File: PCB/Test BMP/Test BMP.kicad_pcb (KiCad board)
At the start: 2 copper layers, 14 x 8 mm, 5 parts, among them J1 4 pins socket, J2 4 pins socket, U1 BMP581

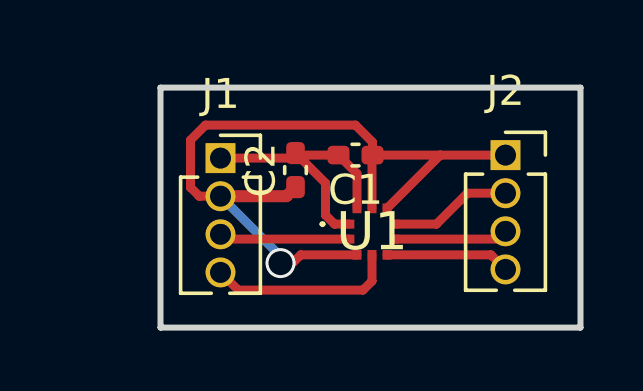
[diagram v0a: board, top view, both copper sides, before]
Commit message: gbr
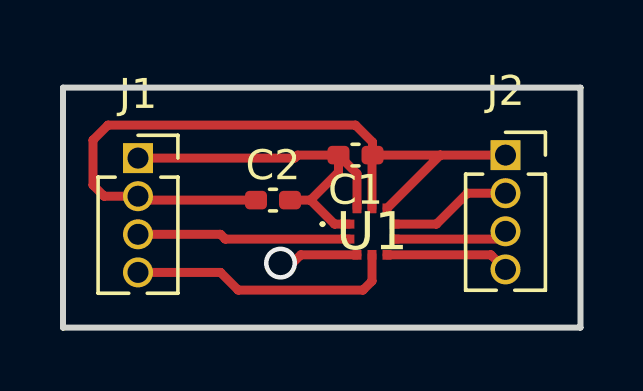
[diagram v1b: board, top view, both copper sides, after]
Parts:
- moved J1 2.75 mm to (135.2, 87.6)
- moved C2 1.25 mm to (139.8, 89.0), turned to 0 degrees
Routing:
- net Net-(J1-Pin_1): track 9.47 -> 13.0 mm
- net Net-(J1-Pin_3): track 4.37 -> 7.12 mm
- net Net-(J1-Pin_4): track 6.29 -> 9.04 mm
- net Net-(J1-Pin_2): track 26.7 -> 29.0 mm
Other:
- board size 14 x 8 mm -> 17.2 x 8 mm
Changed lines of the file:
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@@
 		(filling no)
 		(pcbplotparams
-			(layerselection 0x00000000_00000000_55555555_5755f5ff)
-			(plot_on_all_layers_selection 0x00000000_00000000_00000000_00000000)
+			(layerselection 0x00000000_00000000_55555555_57555555)
+			(plot_on_all_layers_selection 0x00000000_00000000_00000000_02000000)
 			(disableapertmacros no)
 			(usegerberextensions no)
@@
 			(outputformat 1)
 			(mirror no)
-			(drillshape 1)
+			(drillshape 0)
 			(scaleselection 1)
 			(outputdirectory "")
@@
 	(footprint "Capacitor_SMD:C_0402_1005Metric_Pad0.74x0.62mm_HandSolder"
 		(layer "F.Cu")
-		(at 140.5 88 90)
+		(at 139.75 89)
 		(descr "Capacitor SMD 0402 (1005 Metric), square (rectangular) end terminal, IPC-7351 nominal with elongated pad for handsoldering. (Body size source: IPC-SM-782 page 76, https://www.pcb-3d.com/wordpress/wp-content/uploads/ipc-sm-782a_amendment_1_and_2.pdf)")
 		(tags "capacitor handsolder")
 		(property "Reference" "C2"
-			(at 0 -1.16 90)
+			(at 0 -1.16 0)
 			(layer "F.SilkS")
 			(effects
@@
 		)
 		(property "Value" "C"
-			(at 0 1.16 90)
+			(at 0 1.16 0)
 			(layer "F.Fab")
 			(effects
@@
 		)
 		(property "Datasheet" ""
-			(at 0 0 90)
+			(at 0 0 0)
 			(layer "F.Fab")
 			(hide yes)
@@
 		)
 		(property "Description" "Unpolarized capacitor"
-			(at 0 0 90)
+			(at 0 0 0)
 			(layer "F.Fab")
 			(hide yes)
@@
 		)
 		(property "KiLib_Generator" "SMD_2terminal_chip_molded"
-			(at 0 0 90)
+			(at 0 0 0)
 			(layer "F.SilkS")
 			(hide yes)
@@
 		)
 		(fp_text user "${REFERENCE}"
-			(at 0 0 90)
+			(at 0 0 0)
 			(layer "F.Fab")
 			(effects
@@
 		)
 		(pad "1" smd roundrect
-			(at -0.5675 0 90)
+			(at -0.5675 0)
 			(size 0.735 0.62)
 			(layers "F.Cu" "F.Mask" "F.Paste")
@@
 		)
 		(pad "2" smd roundrect
-			(at 0.5675 0 90)
+			(at 0.5675 0)
 			(size 0.735 0.62)
 			(layers "F.Cu" "F.Mask" "F.Paste")
@@
 	(footprint "Bibliotheque_Projet:4 pins socket"
 		(layer "F.Cu")
-		(at 138 87.6)
+		(at 135.25 87.6)
 		(descr "Through hole straight socket strip, 1x04, 1.27mm pitch, single row (from Kicad 4.0.7), script generated")
 		(tags "Through hole socket strip THT 1x04 1.27mm single row")
@@
 	)
 	(gr_rect
-		(start 136 85.25)
+		(start 132.75 85.25)
 		(end 150 93.25)
 		(stroke
@@
 	)
 	(segment
-		(start 140.5675 87.5)
-		(end 140.5 87.4325)
-		(width 0.2)
-		(layer "F.Cu")
-		(net "Net-(J1-Pin_1)")
-	)
-	(segment
-		(start 140.3325 87.6)
-		(end 140.5 87.4325)
-		(width 0.2)
+		(start 141 89)
+		(end 141.9325 88.0675)
+		(width 0.3)
 		(layer "F.Cu")
 		(net "Net-(J1-Pin_1)")
@@
 	)
 	(segment
-		(start 141.5 88.4325)
-		(end 140.5 87.4325)
+		(start 141 89)
+		(end 140.3175 89)
 		(width 0.3)
 		(layer "F.Cu")
@@
 	)
 	(segment
-		(start 138 87.6)
-		(end 140.3325 87.6)
+		(start 140.4675 87.6)
+		(end 135.25 87.6)
 		(width 0.3)
 		(layer "F.Cu")
@@
 	(segment
 		(start 141.8 89.8)
-		(end 141.5 89.5)
+		(end 141 89)
 		(width 0.3)
 		(layer "F.Cu")
@@
 	)
 	(segment
-		(start 141.5 89.5)
-		(end 141.5 88.4325)
+		(start 140.5675 87.5)
+		(end 140.4675 87.6)
+		(width 0.3)
+		(layer "F.Cu")
+		(net "Net-(J1-Pin_1)")
+	)
+	(segment
+		(start 141.9325 88.0675)
+		(end 141.9325 87.5)
 		(width 0.3)
 		(layer "F.Cu")
@@
 	)
 	(segment
+		(start 138 90.14)
+		(end 135.25 90.14)
+		(width 0.3)
+		(layer "F.Cu")
+		(net "Net-(J1-Pin_3)")
+	)
+	(segment
+		(start 142.3 90.3)
+		(end 138.16 90.3)
+		(width 0.3)
+		(layer "F.Cu")
+		(net "Net-(J1-Pin_3)")
+	)
+	(segment
 		(start 138.16 90.3)
 		(end 138 90.14)
-		(width 0.2)
+		(width 0.3)
 		(layer "F.Cu")
 		(net "Net-(J1-Pin_3)")
 	)
 	(segment
-		(start 142.3 90.3)
-		(end 138.16 90.3)
-		(width 0.3)
-		(layer "F.Cu")
-		(net "Net-(J1-Pin_3)")
-	)
-	(segment
-		(start 140.1975 88.87)
-		(end 140.5 88.5675)
-		(width 0.4)
+		(start 133.75 88.5)
+		(end 134.12 88.87)
+		(width 0.3)
 		(layer "F.Cu")
 		(net "Net-(J1-Pin_2)")
@@
 	)
 	(segment
-		(start 143.0675 87.5)
-		(end 143.0675 87.0675)
-		(width 0.3)
-		(layer "F.Cu")
-		(net "Net-(J1-Pin_2)")
-	)
-	(segment
-		(start 137 87)
-		(end 137 88.577106)
-		(width 0.3)
-		(layer "F.Cu")
-		(net "Net-(J1-Pin_2)")
-	)
-	(segment
-		(start 137.5 86.5)
-		(end 137 87)
+		(start 143.0675 87.0675)
+		(end 142.5 86.5)
+		(width 0.3)
+		(layer "F.Cu")
+		(net "Net-(J1-Pin_2)")
+	)
+	(segment
+		(start 134.25 86.5)
+		(end 133.75 87)
+		(width 0.3)
+		(layer "F.Cu")
+		(net "Net-(J1-Pin_2)")
+	)
+	(segment
+		(start 133.75 87)
+		(end 133.75 88.5)
 		(width 0.3)
 		(layer "F.Cu")
@@
 	)
 	(segment
+		(start 142.5 86.5)
+		(end 134.25 86.5)
+		(width 0.3)
+		(layer "F.Cu")
+		(net "Net-(J1-Pin_2)")
+	)
+	(segment
 		(start 145.325 87.5)
 		(end 147.5 87.5)
@@
 	)
 	(segment
-		(start 137.292894 88.87)
-		(end 138 88.87)
-		(width 0.3)
+		(start 135.38 89)
+		(end 135.25 88.87)
+		(width 0.2)
 		(layer "F.Cu")
 		(net "Net-(J1-Pin_2)")
@@
 	)
 	(segment
-		(start 142.5 86.5)
-		(end 137.5 86.5)
-		(width 0.3)
-		(layer "F.Cu")
-		(net "Net-(J1-Pin_2)")
-	)
-	(segment
-		(start 137 88.577106)
-		(end 137.292894 88.87)
-		(width 0.3)
-		(layer "F.Cu")
-		(net "Net-(J1-Pin_2)")
-	)
-	(segment
 		(start 140.675 90.825)
 		(end 142.55 90.825)
@@
 	)
 	(segment
-		(start 143.0675 87.0675)
-		(end 142.5 86.5)
-		(width 0.3)
-		(layer "F.Cu")
-		(net "Net-(J1-Pin_2)")
-	)
-	(segment
-		(start 138 88.87)
-		(end 140.1975 88.87)
-		(width 0.4)
+		(start 134.12 88.87)
+		(end 135.25 88.87)
+		(width 0.3)
+		(layer "F.Cu")
+		(net "Net-(J1-Pin_2)")
+	)
+	(segment
+		(start 139.1825 89)
+		(end 135.38 89)
+		(width 0.3)
+		(layer "F.Cu")
+		(net "Net-(J1-Pin_2)")
+	)
+	(segment
+		(start 143.0675 87.5)
+		(end 143.0675 87.0675)
+		(width 0.3)
 		(layer "F.Cu")
 		(net "Net-(J1-Pin_2)")
@@
 	(via
 		(at 140 91.1)
-		(size 1)
+		(size 1.1)
 		(drill 0.8)
 		(layers "F.Cu" "B.Cu")
@@
 	)
 	(segment
-		(start 140 90.87)
-		(end 138 88.87)
-		(width 0.3)
-		(layer "B.Cu")
-		(net "Net-(J1-Pin_2)")
-	)
-	(segment
+		(start 138 91.41)
+		(end 135.25 91.41)
+		(width 0.3)
+		(layer "F.Cu")
+		(net "Net-(J1-Pin_4)")
+	)
+	(segment
